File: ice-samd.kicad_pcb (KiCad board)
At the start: 2 copper layers, 50.8 x 22.9 mm, 34 parts, among them IC1 ADXL345, J1 Conn_Battery, J2 USB_B_Micro, J3 Conn_Left, J4 Conn_Right, U1 SPX3819M5-L-3-3, U2 ATSAMD21G18A-AUT, U3 MCP73831-2-OT, U4 ATECC608A-MAHDA, Y1 32.768

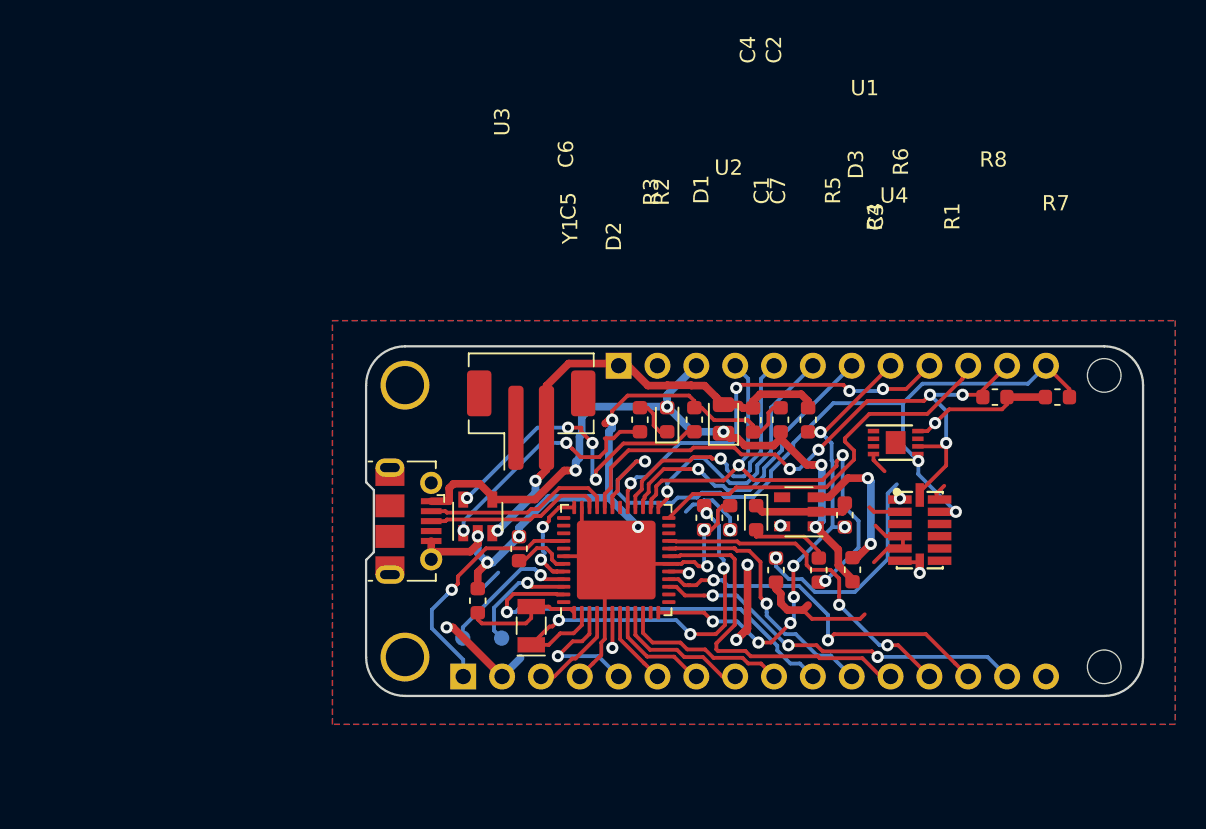
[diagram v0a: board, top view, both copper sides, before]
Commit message: Updated LED locations
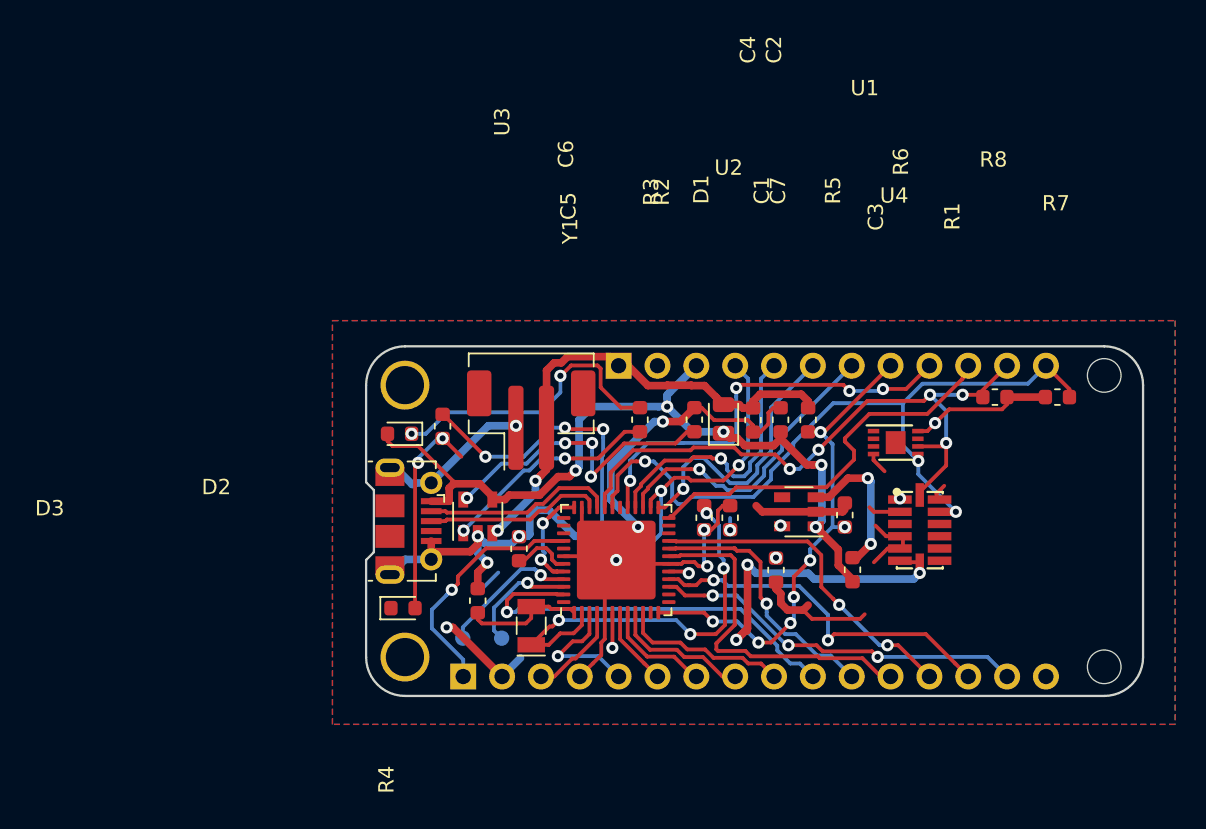
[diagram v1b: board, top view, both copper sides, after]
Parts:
- moved R4 26.3 mm to (132.0, 86.5), turned to 270 degrees
- moved D3 23.8 mm to (129.4, 98.4), turned to 0 degrees
- moved D2 17.5 mm to (129.2, 87.0), turned to 180 degrees
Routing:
- net Net-(D2-Pad1): track 2.87 -> 19.3 mm, vias 0 -> 2
- net GND: track 97.5 -> 109.2 mm, vias 7 -> 9
- net Net-(D3-Pad2): track 5.38 -> 14.0 mm, vias 0 -> 2
- net /D13: track 33.3 -> 41.8 mm, vias 3 -> 5
- net +3V3: track 55.8 -> 49.3 mm
- net VBUS: track 46.0 -> 52.1 mm
- net /SDA: track 53.0 -> 49.7 mm
- net Net-(R2-Pad1): track 21.5 -> 20.2 mm
- net +BATT: track 32.0 -> 33.2 mm
- net Net-(R3-Pad2): track 16.1 -> 14.9 mm
- net /D6: track 26.7 -> 27.8 mm
